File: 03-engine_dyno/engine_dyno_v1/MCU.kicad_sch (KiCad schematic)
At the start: 4 parts, among them IC1 TEENSY_4.1, P1 J1B1211CCD, U6 Teensy4.1

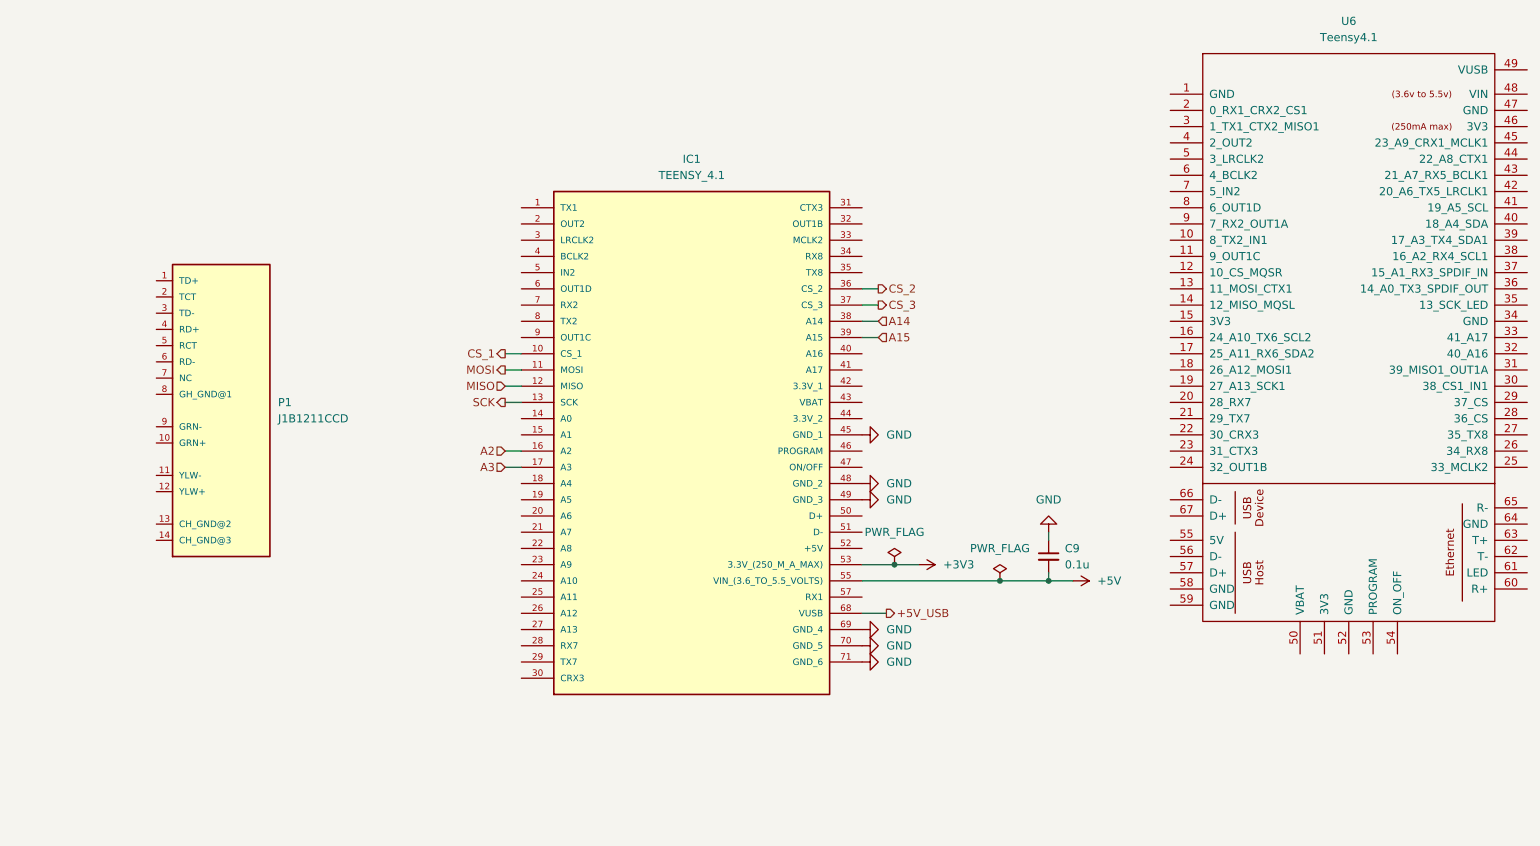
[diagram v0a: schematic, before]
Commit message: new transducer
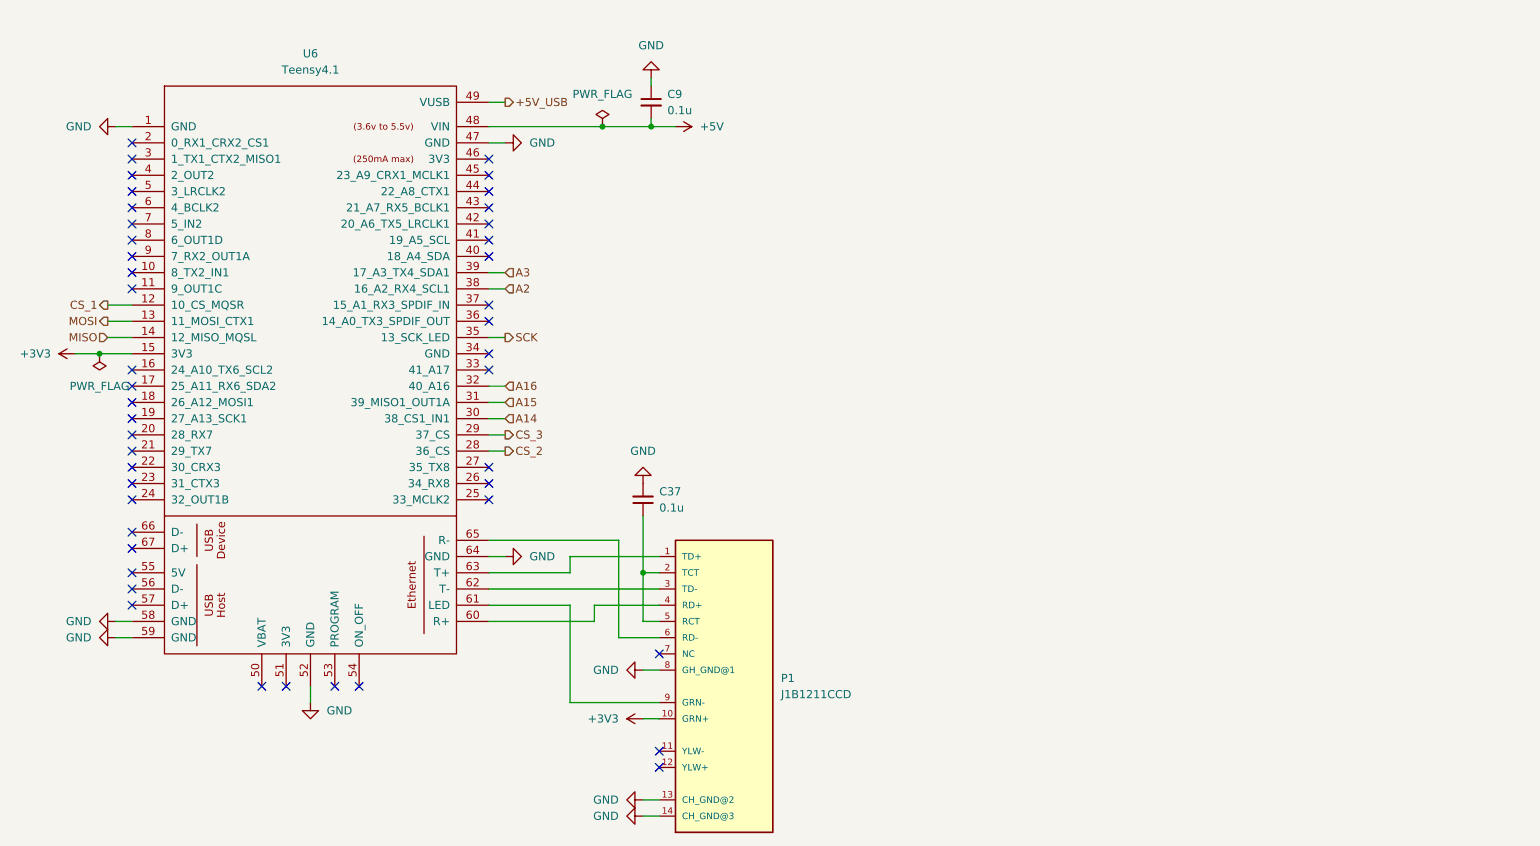
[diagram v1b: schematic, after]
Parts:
- removed IC1: TEENSY_4.1, engine_dyno:TEENSY41, symbol TEENSY_4.1:TEENSY_4.1
- added C37: 0.1u, symbol Device:C_Small
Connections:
- net +3V3: now also P1.10 (GRN+), U6.15 (3V3)
- net +5V: now also U6.48 (VIN)
- net +5V_USB: now also U6.49 (VUSB)
- net A14: now also U6.30 (38_CS1_IN1)
- net A15: now also U6.31 (39_MISO1_OUT1A)
- net A2: now also U6.38 (16_A2_RX4_SCL1)
- net A3: now also U6.39 (17_A3_TX4_SDA1)
- net CS_1: now also U6.12 (10_CS_MQSR)
- net CS_2: now also U6.28 (36_CS)
- net CS_3: now also U6.29 (37_CS)
- net GND: now also P1.13 (CH_GND@2), P1.14 (CH_GND@3), P1.8 (GH_GND@1), U6.1 (GND), U6.47 (GND), U6.52 (GND), U6.58 (GND), U6.59 (GND), U6.64 (GND), C37.2
- net MISO: now also U6.14 (12_MISO_MQSL)
- net MOSI: now also U6.13 (11_MOSI_CTX1)
- net SCK: now also U6.35 (13_SCK_LED)
- net at P1.1 (TD+): now also U6.63 (T+)
- net at P1.2 (TCT): now also P1.5 (RCT), C37.1
- net at P1.3 (TD-): now also U6.62 (T-)
- net at P1.4 (RD+): now also U6.60 (R+)
- net at P1.6 (RD-): now also U6.65 (R-)
- net at P1.9 (GRN-): now also U6.61 (LED)
- net A16: now reaches U6.32 (40_A16)
- no-connect marks 0 -> 45
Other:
- moved on the sheet: C9, P1, U6

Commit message: beginnings of a pcb
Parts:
- C37, C9: footprint (none) -> Capacitor_SMD:C_0402_1005Metric
- U6: footprint 22XT_Main:Teensy41 -> engine_dyno:Teensy41
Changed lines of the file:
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@@
 			)
 		)
-		(property "Footprint" ""
+		(property "Footprint" "Capacitor_SMD:C_0402_1005Metric"
 			(at 134.62 104.14 0)
 			(effects
@@
 			)
 		)
-		(property "Footprint" ""
+		(property "Footprint" "Capacitor_SMD:C_0402_1005Metric"
 			(at 135.89 41.91 0)
 			(effects
@@
 			)
 		)
-		(property "Footprint" "22XT_Main:Teensy41"
+		(property "Footprint" "engine_dyno:Teensy41"
 			(at 72.39 90.17 0)
 			(effects
